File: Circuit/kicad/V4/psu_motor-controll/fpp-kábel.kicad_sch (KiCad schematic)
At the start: 1 part, among them J5 Conn_01x60_MountingPin

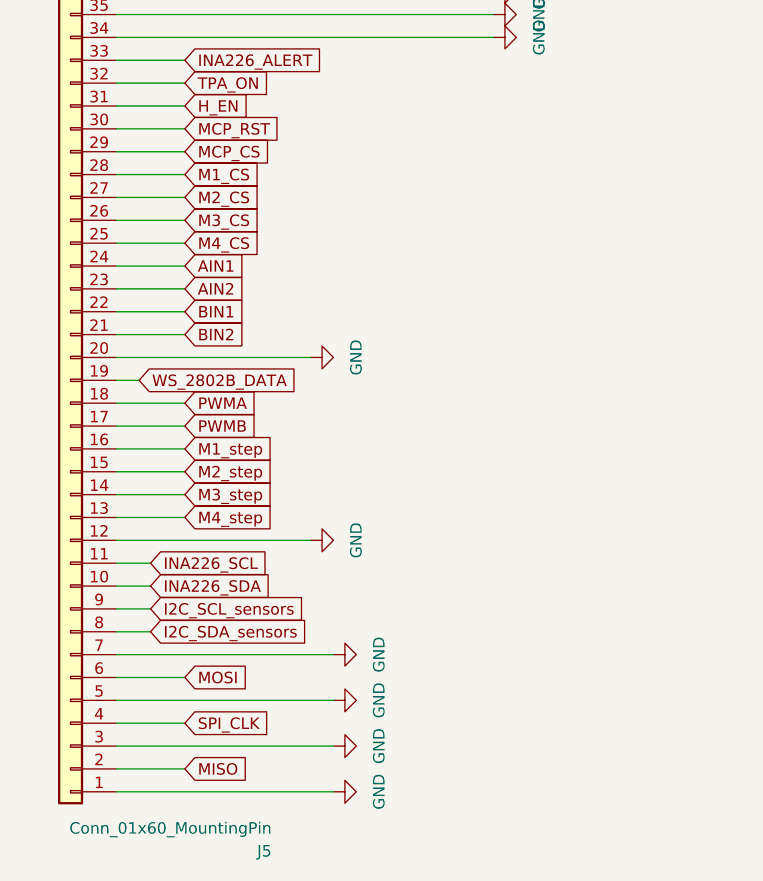
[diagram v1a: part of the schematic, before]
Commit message: kicad psu pcb finish psu
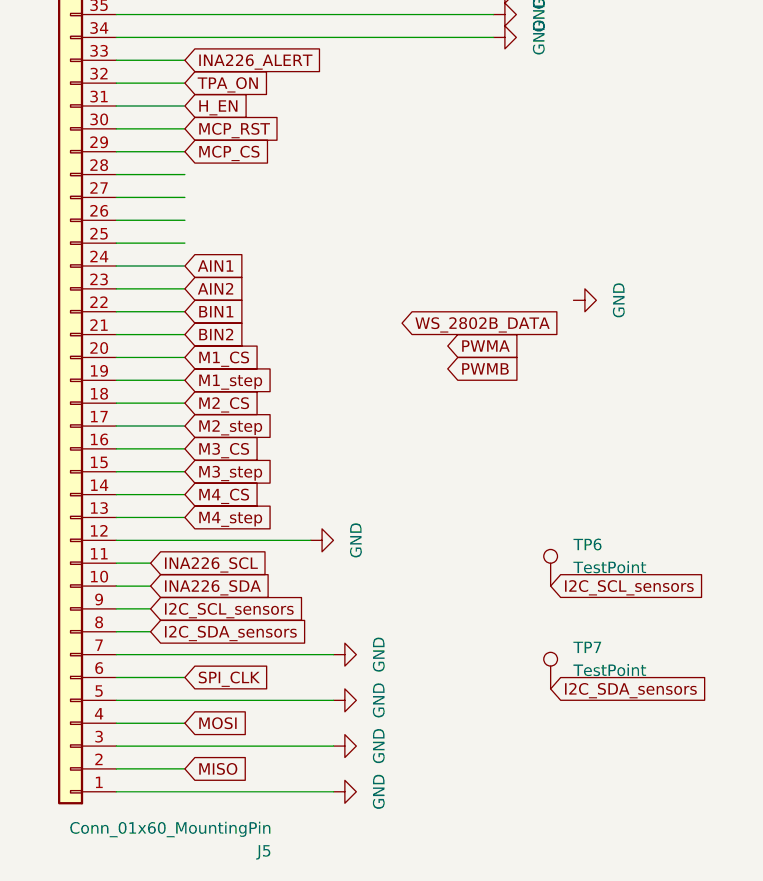
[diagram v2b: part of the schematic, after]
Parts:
- added TP6, TP7: TestPoint, TestPoint:TestPoint_Pad_D1.0mm, symbol Connector:TestPoint
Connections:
- net GND: no longer J5.20 (Pin_20)
- net I2C_SCL_sensors: now also TP6.1
- net I2C_SDA_sensors: now also TP7.1
- net M1_CS: now also J5.20 (Pin_20); no longer J5.28 (Pin_28)
- net M1_step: now also J5.19 (Pin_19); no longer J5.16 (Pin_16)
- net M2_CS: now also J5.18 (Pin_18); no longer J5.27 (Pin_27)
- net M2_step: now also J5.17 (Pin_17); no longer J5.15 (Pin_15)
- net M3_CS: now also J5.16 (Pin_16); no longer J5.26 (Pin_26)
- net M3_step: now also J5.15 (Pin_15); no longer J5.14 (Pin_14)
- net M4_CS: now also J5.14 (Pin_14); no longer J5.25 (Pin_25)
- net MOSI: now also J5.4 (Pin_4); no longer J5.6 (Pin_6)
- net PWMA: no longer J5.18 (Pin_18)
- net PWMB: no longer J5.17 (Pin_17)
- net SPI_CLK: now also J5.6 (Pin_6); no longer J5.4 (Pin_4)
- net WS_2802B_DATA: no longer J5.19 (Pin_19)

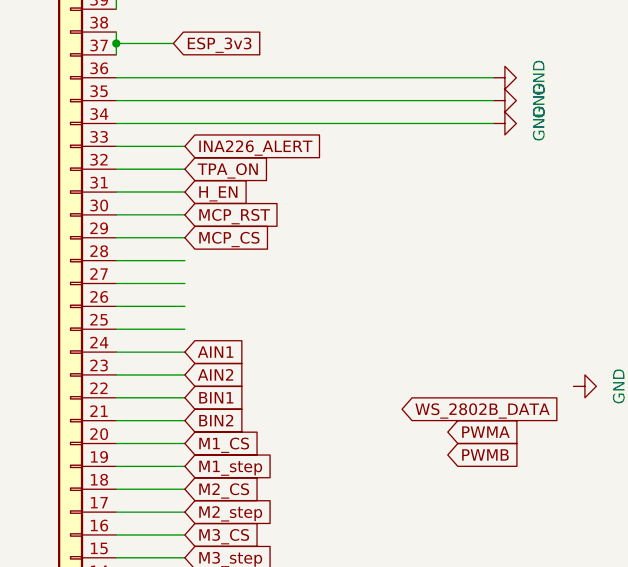
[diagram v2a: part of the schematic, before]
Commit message: psu pcb update
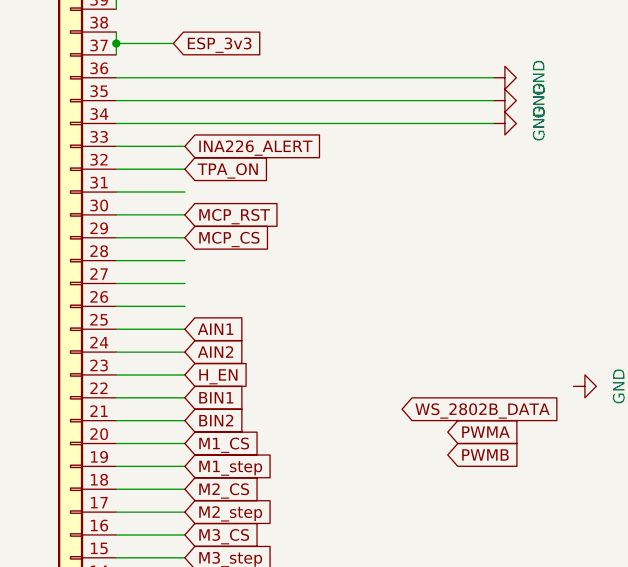
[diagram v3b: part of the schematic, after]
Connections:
- net AIN1: now also J5.25 (Pin_25); no longer J5.24 (Pin_24)
- net AIN2: now also J5.24 (Pin_24); no longer J5.23 (Pin_23)
- net H_EN: now also J5.23 (Pin_23); no longer J5.31 (Pin_31)
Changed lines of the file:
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@@
+		)
+	)
+	(global_label "AIN1"
+		(shape input)
+		(at 31.75 114.3 0)
+		(fields_autoplaced yes)
+		(effects
+			(font
+				(size 1.27 1.27)
+			)
+			(justify left)
+		)
+		(property "Intersheetrefs" "${INTERSHEET_REFS}"
+			(at 39.0637 114.3 0)
+			(effects
+				(font
+					(size 1.27 1.27)
+				)
+				(justify left)
+				(hide yes)
+			)
 		)
 	)
@@
 		)
 	)
+	(global_label "H_EN"
+		(shape input)
+		(at 31.75 119.38 0)
+		(fields_autoplaced yes)
+		(effects
+			(font
+				(size 1.27 1.27)
+			)
+			(justify left)
+		)
+		(property "Intersheetrefs" "${INTERSHEET_REFS}"
+			(at 39.6079 119.38 0)
+			(effects
+				(font
+					(size 1.27 1.27)
+				)
+				(justify left)
+				(hide yes)
+			)
+		)
+	)
 	(global_label "MOSI"
 		(shape input)
@@
 		)
 	)
+	(global_label "AIN2"
+		(shape input)
+		(at 31.75 116.84 0)
+		(fields_autoplaced yes)
+		(effects
+			(font
+				(size 1.27 1.27)
+			)
+			(justify left)
+		)
+		(property "Intersheetrefs" "${INTERSHEET_REFS}"
+			(at 39.0637 116.84 0)
+			(effects
+				(font
+					(size 1.27 1.27)
+				)
+				(justify left)
+				(hide yes)
+			)
+		)
+	)
 	(global_label "M2_step"
 		(shape input)
@@
 		)
 	)
-	(global_label "H_EN"
-		(shape input)
-		(at 31.75 99.06 0)
-		(fields_autoplaced yes)
-		(effects
-			(font
-				(size 1.27 1.27)
-			)
-			(justify left)
-		)
-		(property "Intersheetrefs" "${INTERSHEET_REFS}"
-			(at 39.6079 99.06 0)
-			(effects
-				(font
-					(size 1.27 1.27)
-				)
-				(justify left)
-				(hide yes)
-			)
-		)
-	)
 	(global_label "RPI_5V"
 		(shape input)
@@
 		)
 	)
-	(global_label "AIN2"
-		(shape input)
-		(at 31.75 119.38 0)
-		(fields_autoplaced yes)
-		(effects
-			(font
-				(size 1.27 1.27)
-			)
-			(justify left)
-		)
-		(property "Intersheetrefs" "${INTERSHEET_REFS}"
-			(at 39.0637 119.38 0)
-			(effects
-				(font
-					(size 1.27 1.27)
-				)
-				(justify left)
-				(hide yes)
-			)
-		)
-	)
 	(global_label "ESP_5v"
 		(shape input)
@@
 			(effects
 				(font
-					(size 1.27 1.27)
-				)
-				(justify left)
-				(hide yes)
-			)
-		)
-	)
-	(global_label "AIN1"
-		(shape input)
-		(at 31.75 116.84 0)
-		(fields_autoplaced yes)
-		(effects
-			(font
-				(size 1.27 1.27)
-			)
-			(justify left)
-		)
-		(property "Intersheetrefs" "${INTERSHEET_REFS}"
-			(at 39.0637 116.84 0)
-			(effects
-				(font

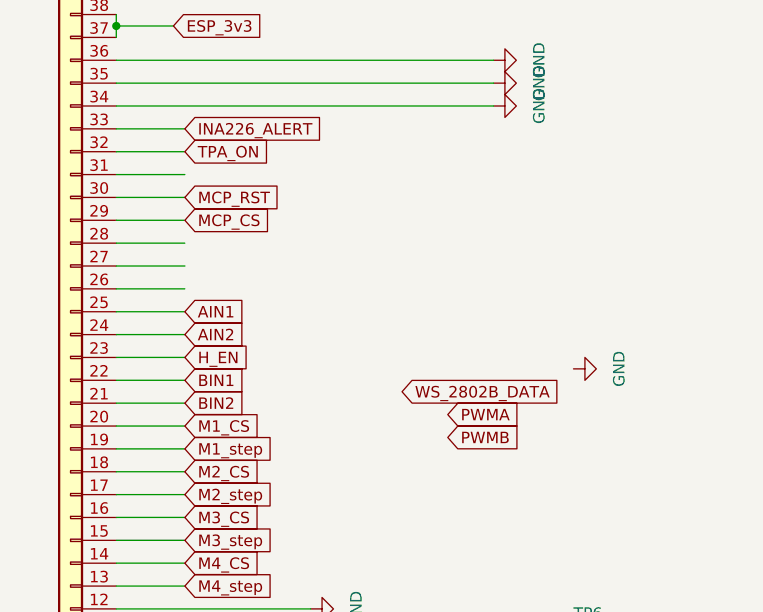
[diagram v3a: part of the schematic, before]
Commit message: kicad FINISH PSU PCB
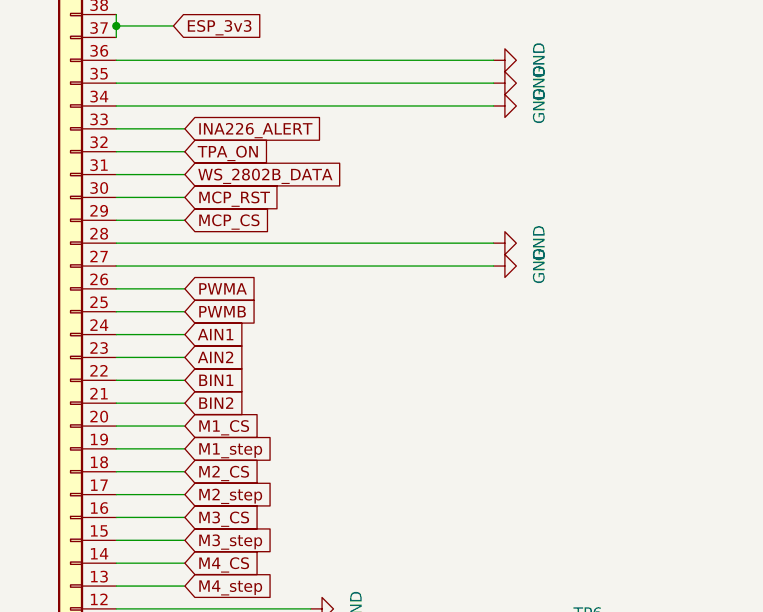
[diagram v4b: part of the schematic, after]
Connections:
- net H_EN is gone; now on net AIN2: J5.23 (Pin_23)
- net AIN1: now also J5.24 (Pin_24); no longer J5.25 (Pin_25)
- net AIN2: no longer J5.24 (Pin_24)
- net GND: now also J5.27 (Pin_27), J5.28 (Pin_28)
- net PWMA: now also J5.26 (Pin_26)
- net PWMB: now also J5.25 (Pin_25)
- net WS_2802B_DATA: now also J5.31 (Pin_31)

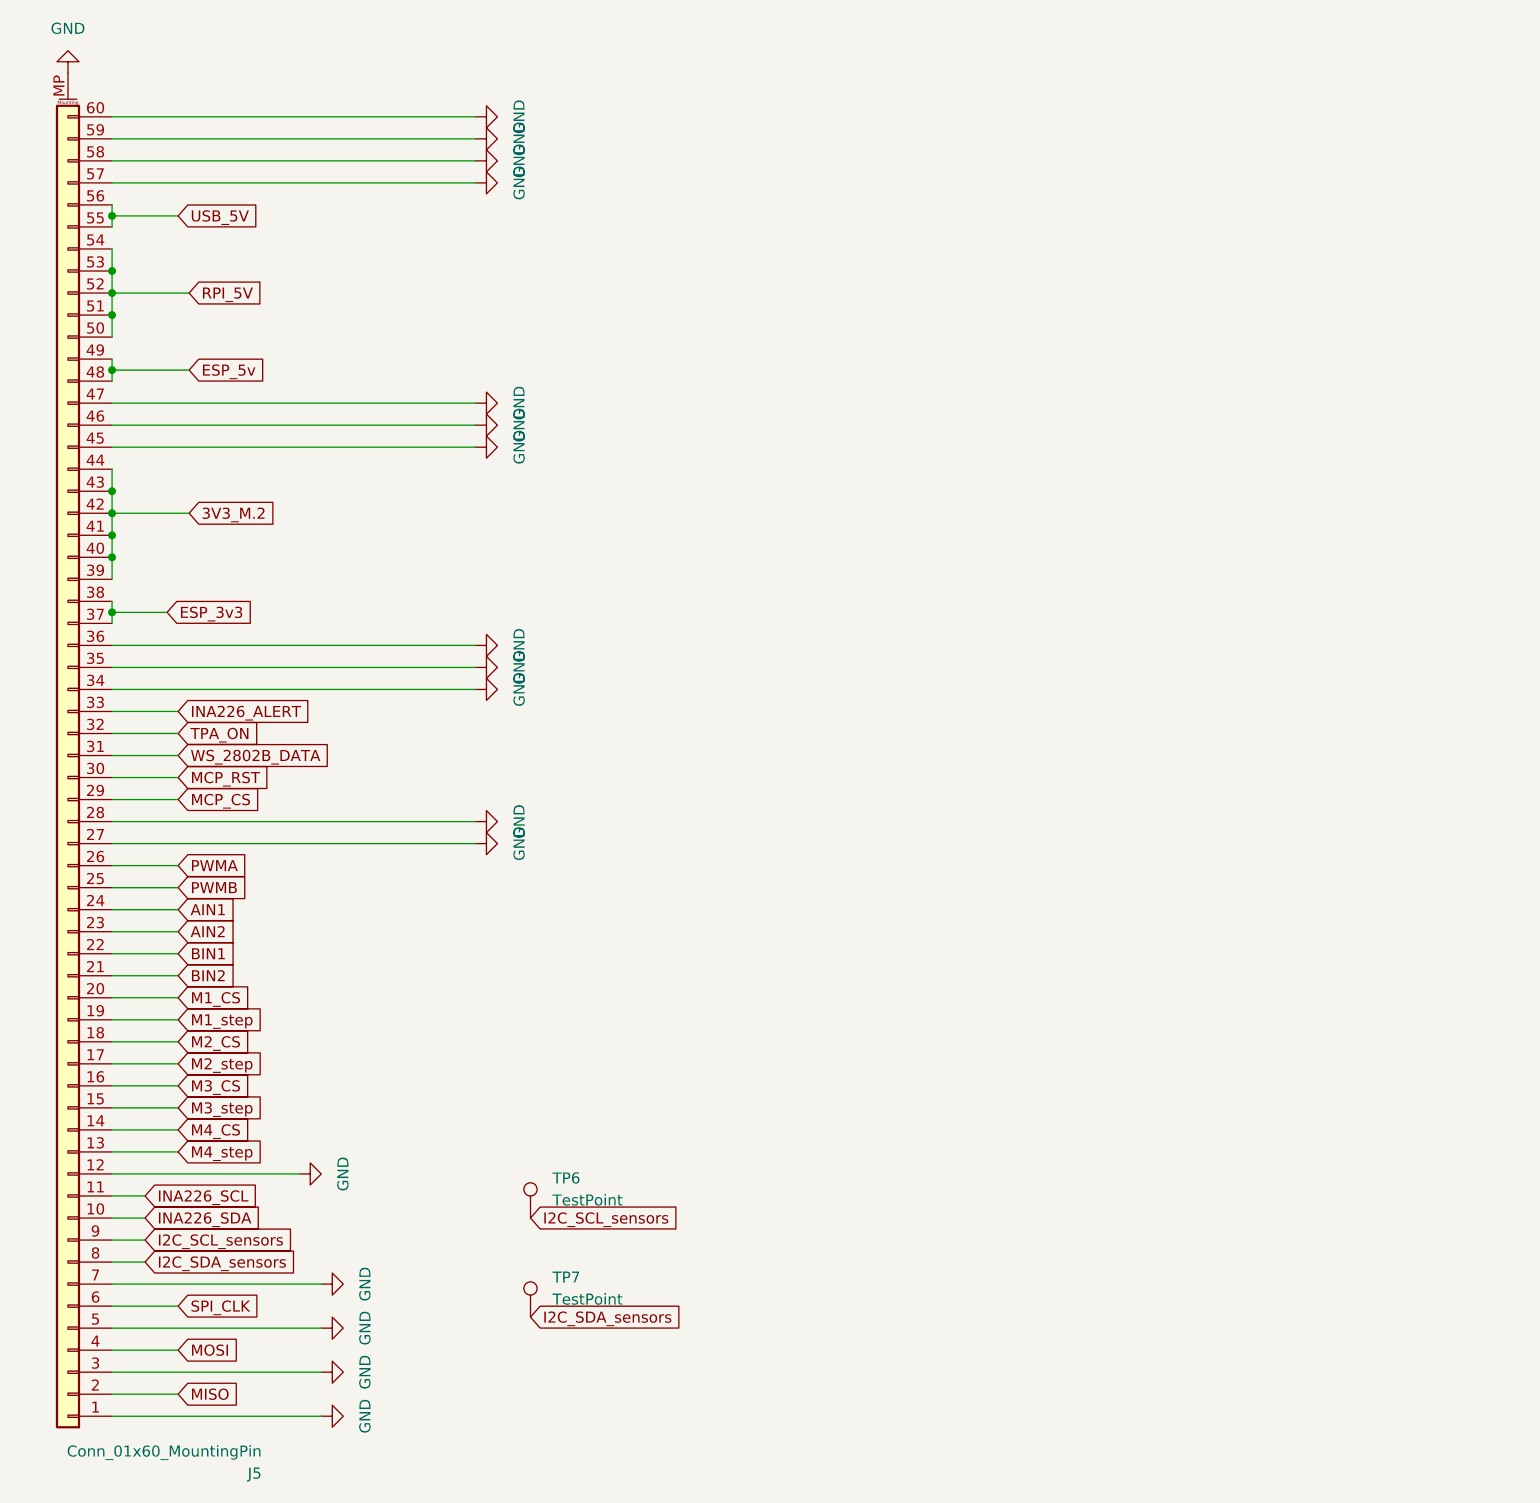
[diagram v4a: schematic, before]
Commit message: PSU bugfixes
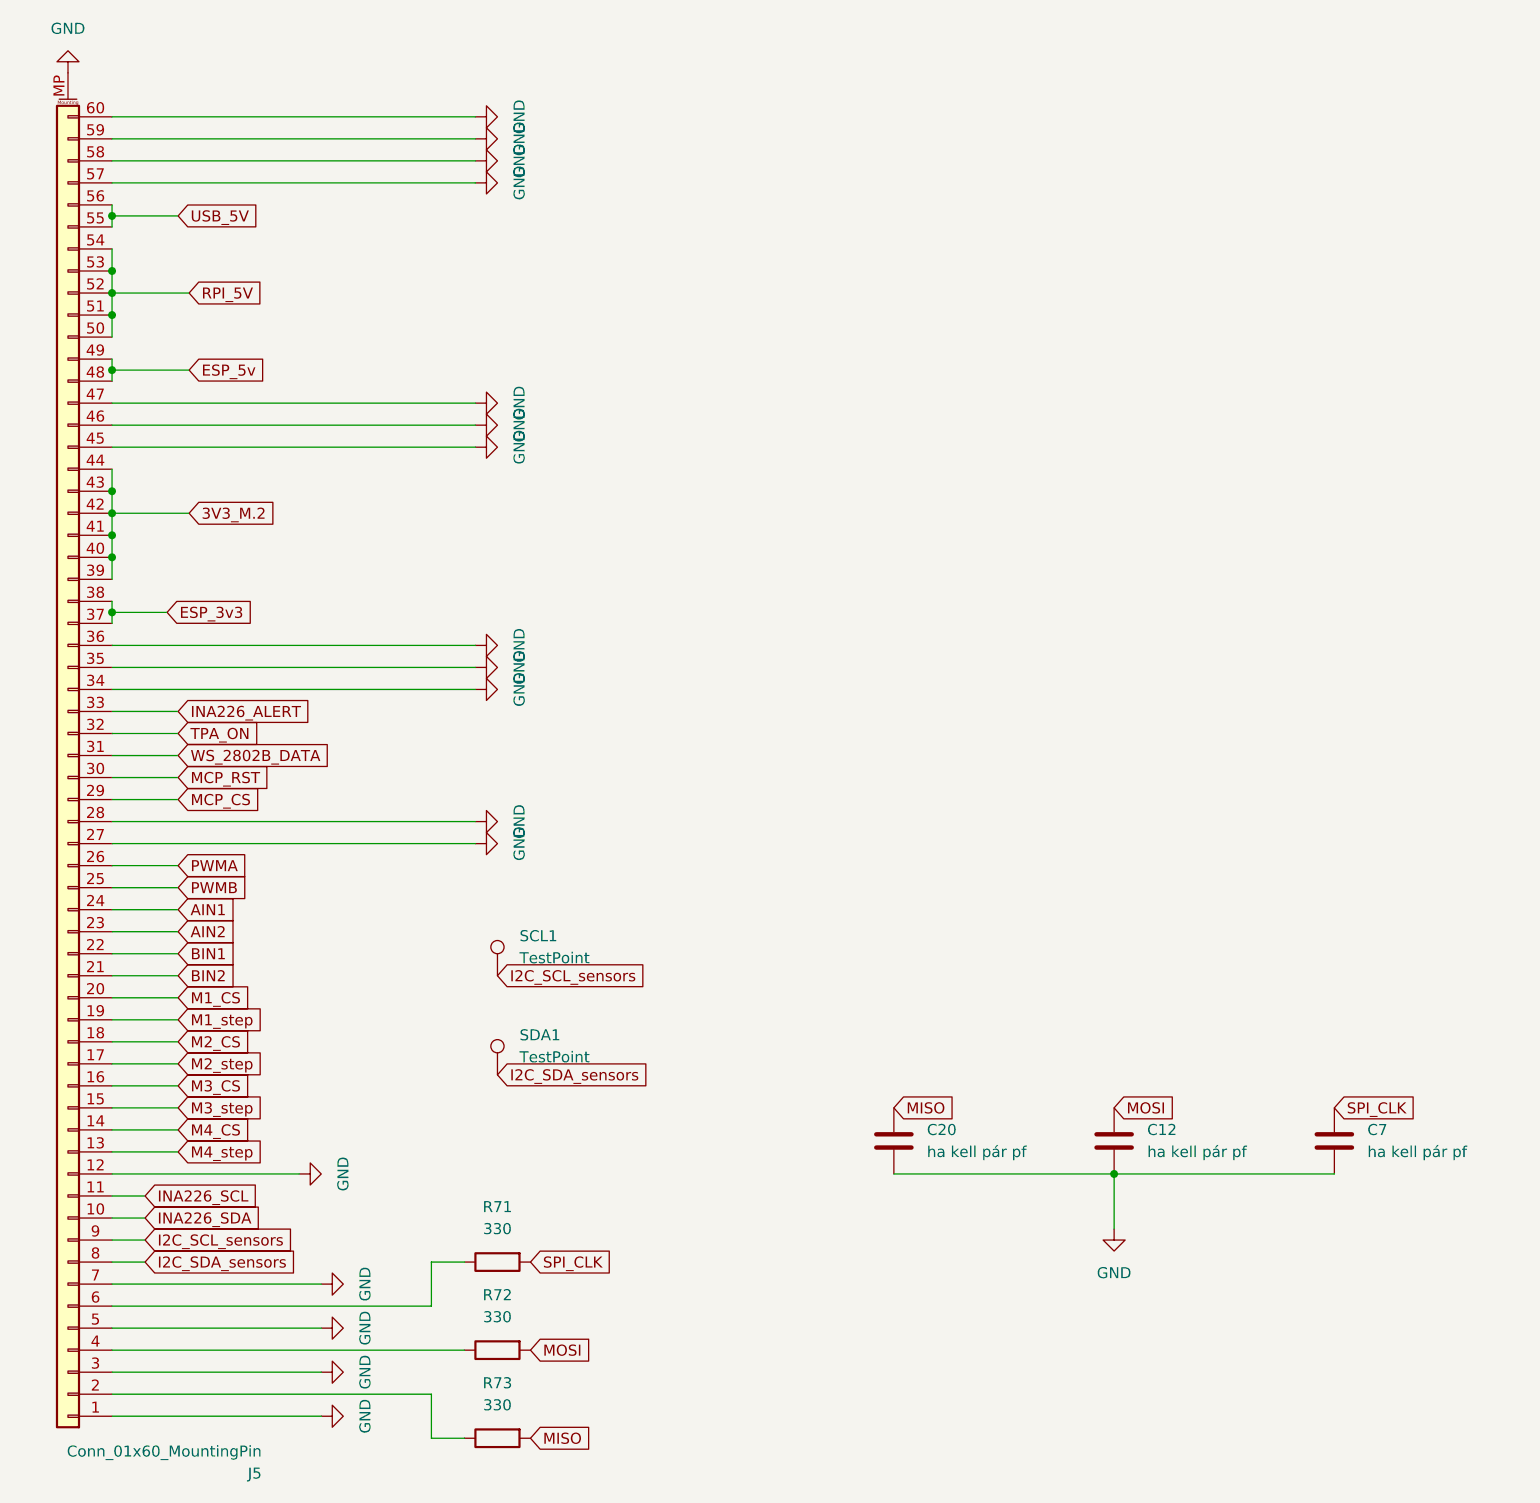
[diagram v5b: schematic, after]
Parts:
- added C12, C20, C7: ha kell pár pf, Capacitor_SMD:C_0805_2012Metric, symbol Device:C
- added R71, R72, R73: 330, Resistor_SMD:R_0805_2012Metric, symbol Device:R
- renumbered TP6 to SCL1, TP7 to SDA1
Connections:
- net GND: now also C12.2, C20.2, C7.2
- net MISO: now also C20.1, R73.2; no longer J5.2 (Pin_2)
- net MOSI: now also C12.1, R72.2; no longer J5.4 (Pin_4)
- net SPI_CLK: now also C7.1, R71.2; no longer J5.6 (Pin_6)
- new net: J5.4 (Pin_4), R72.1
- new net: J5.2 (Pin_2), R73.1
- new net: J5.6 (Pin_6), R71.1
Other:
- moved on the sheet: SCL1, SDA1
